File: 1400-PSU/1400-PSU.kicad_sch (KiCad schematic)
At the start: 42 parts, among them J1 Battery, J2 Jack-DC, J3 MAINBOARD_OUT, Q1 IRF9540N, SW1 SW_DPST, U3 LM7805_TO220, U4 LM340T-12, U5 N7812-1PH

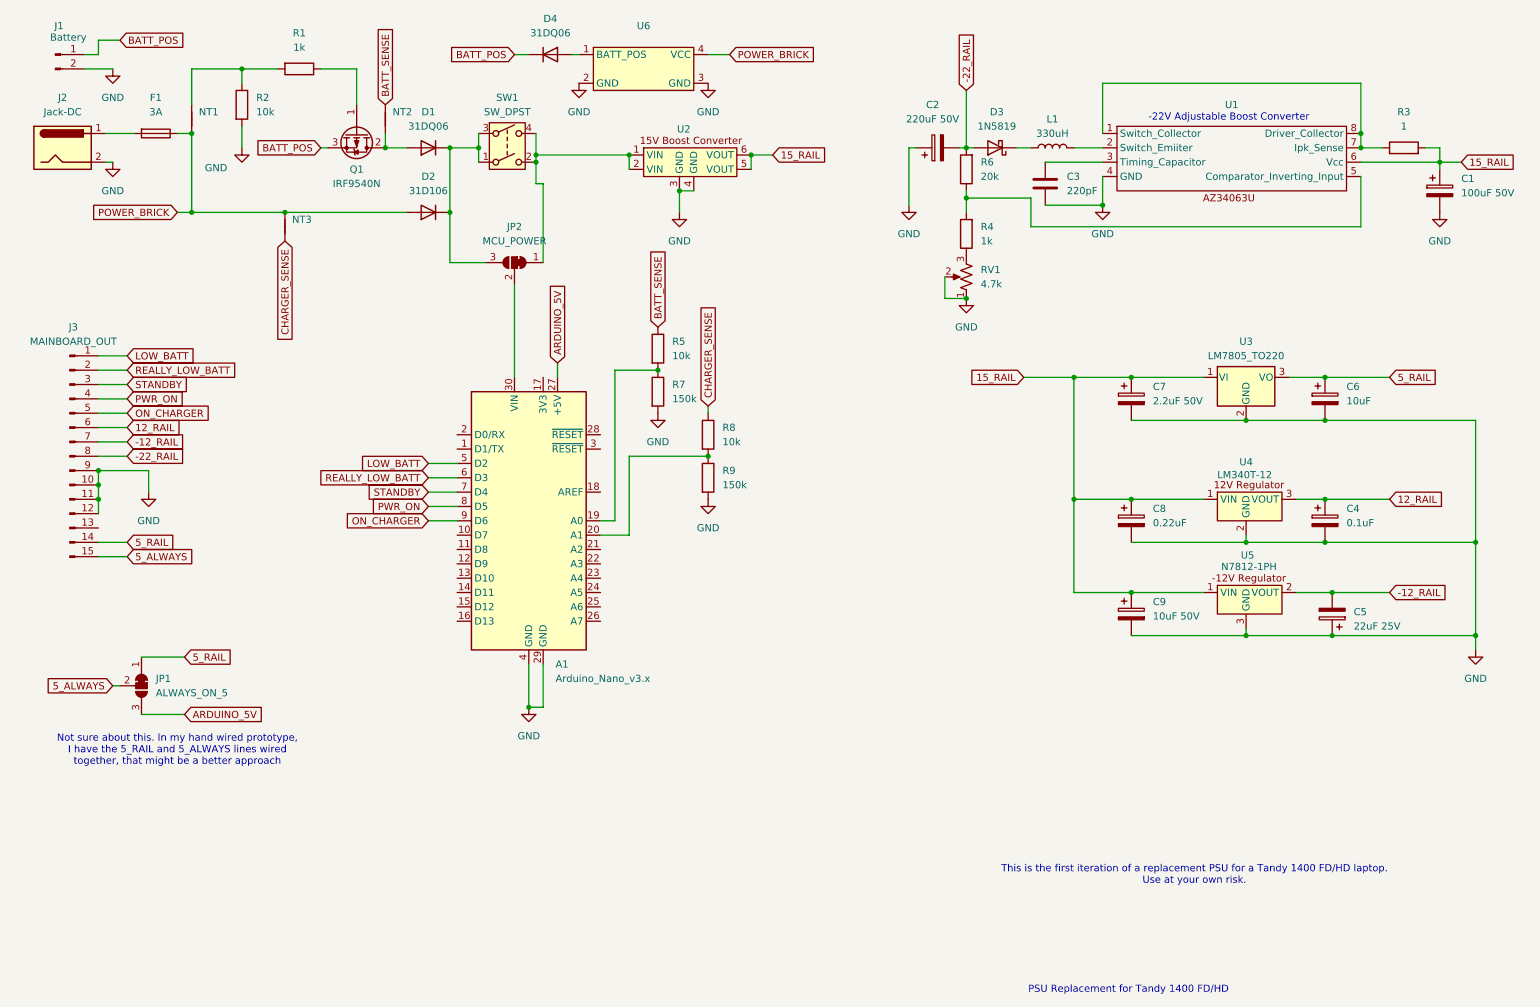
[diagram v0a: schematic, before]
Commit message: Updating for next board revision.
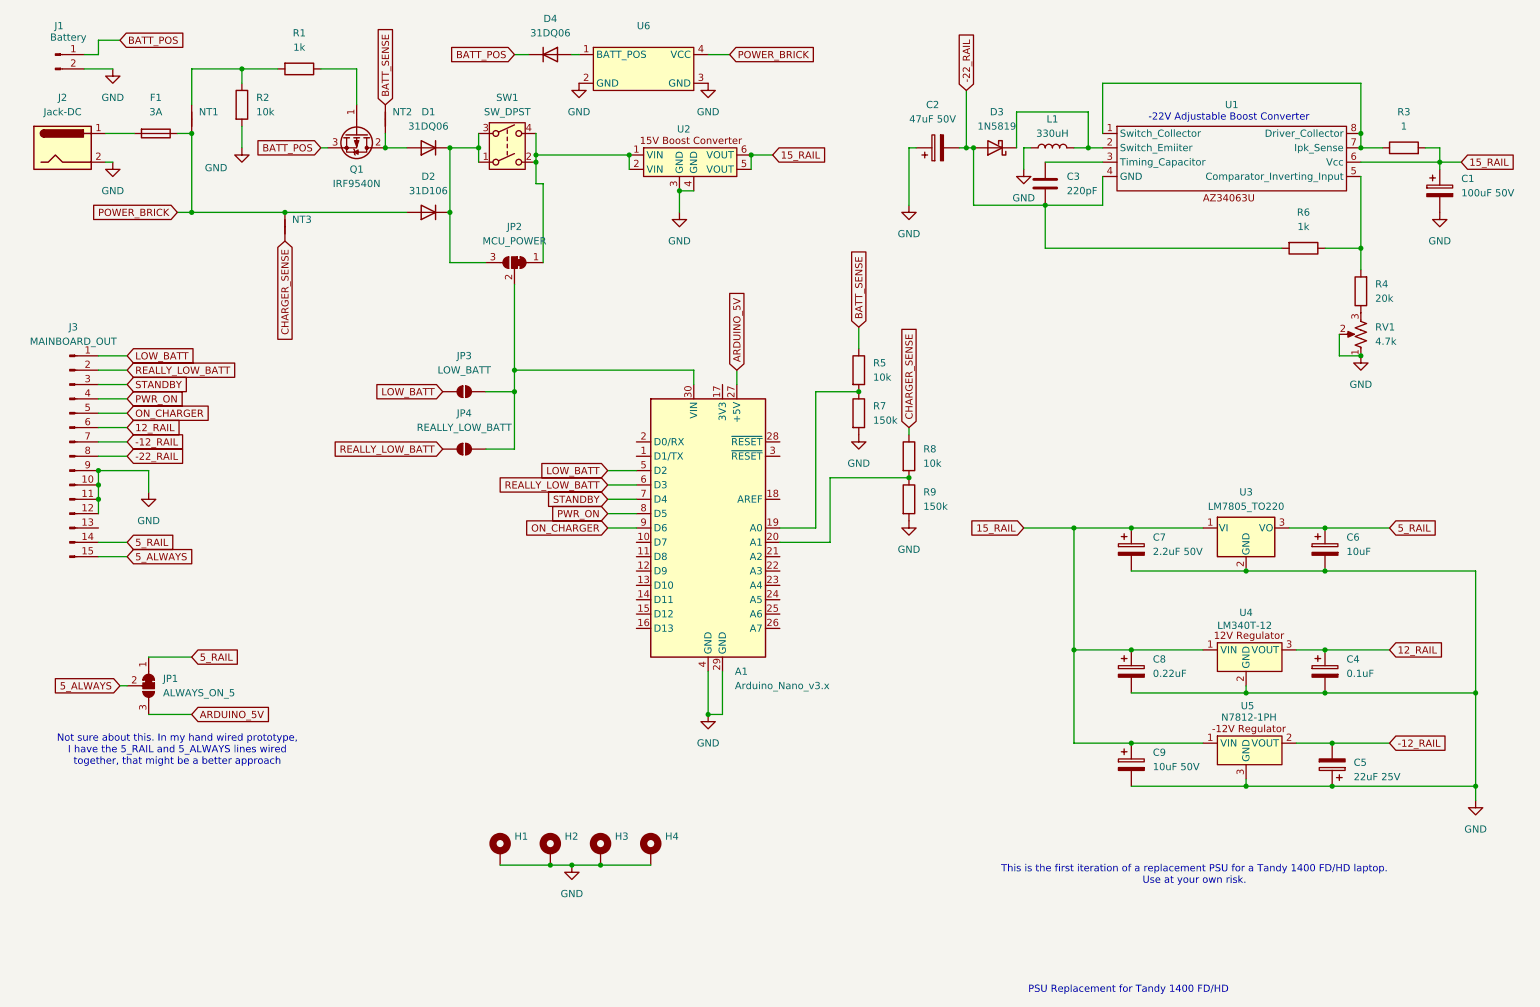
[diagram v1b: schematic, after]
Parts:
- added H1, H2, H3, H4: ~, MountingHole:MountingHole_3.5mm_Pad_TopBottom, symbol Mechanical:MountingHole_Pad
- added JP3: LOW_BATT, Jumper:SolderJumper-2_P1.3mm_Open_RoundedPad1.0x1.5mm, symbol Jumper:SolderJumper_2_Open
- added JP4: REALLY_LOW_BATT, Jumper:SolderJumper-2_P1.3mm_Open_RoundedPad1.0x1.5mm, symbol Jumper:SolderJumper_2_Open
- C2: value 220uF 50V -> 47uF 50V
- D1: footprint Diode_THT:D_DO-41_SOD81_P10.16mm_Horizontal -> Diode_THT:D_DO-201AD_P5.08mm_Vertical_AnodeUp
- D2: footprint Diode_THT:D_DO-41_SOD81_P10.16mm_Horizontal -> Diode_THT:D_DO-201AD_P5.08mm_Vertical_KathodeUp
- D4: footprint Diode_THT:D_DO-41_SOD81_P10.16mm_Horizontal -> Diode_THT:D_DO-201AD_P12.70mm_Horizontal
- R4: value 1k -> 20k
- R6: value 20k -> 1k
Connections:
- net -22_RAIL: now also C3.2, U1.4 (GND)
- net GND: now also L1.1, H1.1, H2.1, H3.1, H4.1; no longer C3.2, U1.4 (GND)
- net LOW_BATT: now also JP3.1 (A)
- net REALLY_LOW_BATT: now also JP4.1 (A)
- net at L1.2, U1.2 (Switch_Emiiter): now also D3.1 (K)
- net at A1.30 (VIN), JP2.2 (C): now also JP3.2 (B), JP4.2 (B)
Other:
- moved on the sheet: A1, C4, C5, C6, C7, C8, C9, JP1, R4, R5, R6, R7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
